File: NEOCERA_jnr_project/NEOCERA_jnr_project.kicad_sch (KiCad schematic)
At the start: 2 parts, among them J4 DB25_Receptacle_MountingHoles, J5 DA15_Receptacle_MountingHoles

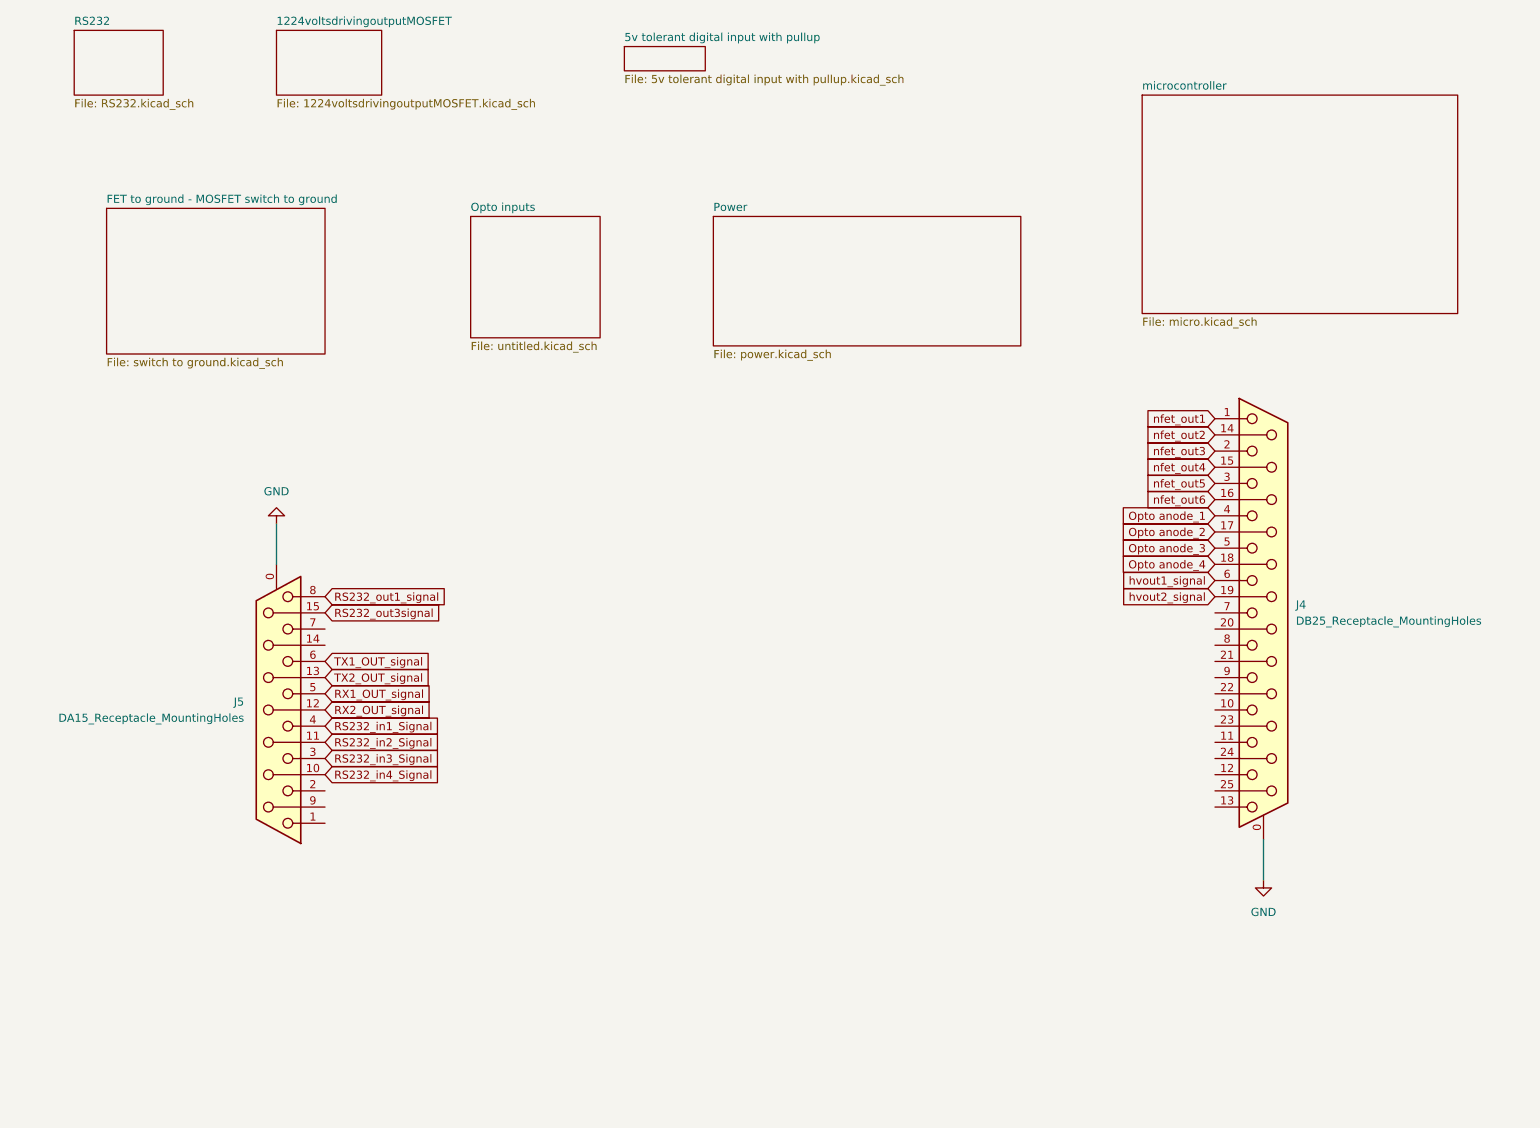
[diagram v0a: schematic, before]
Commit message: bunch of edits
bunch of edits were done including DB37
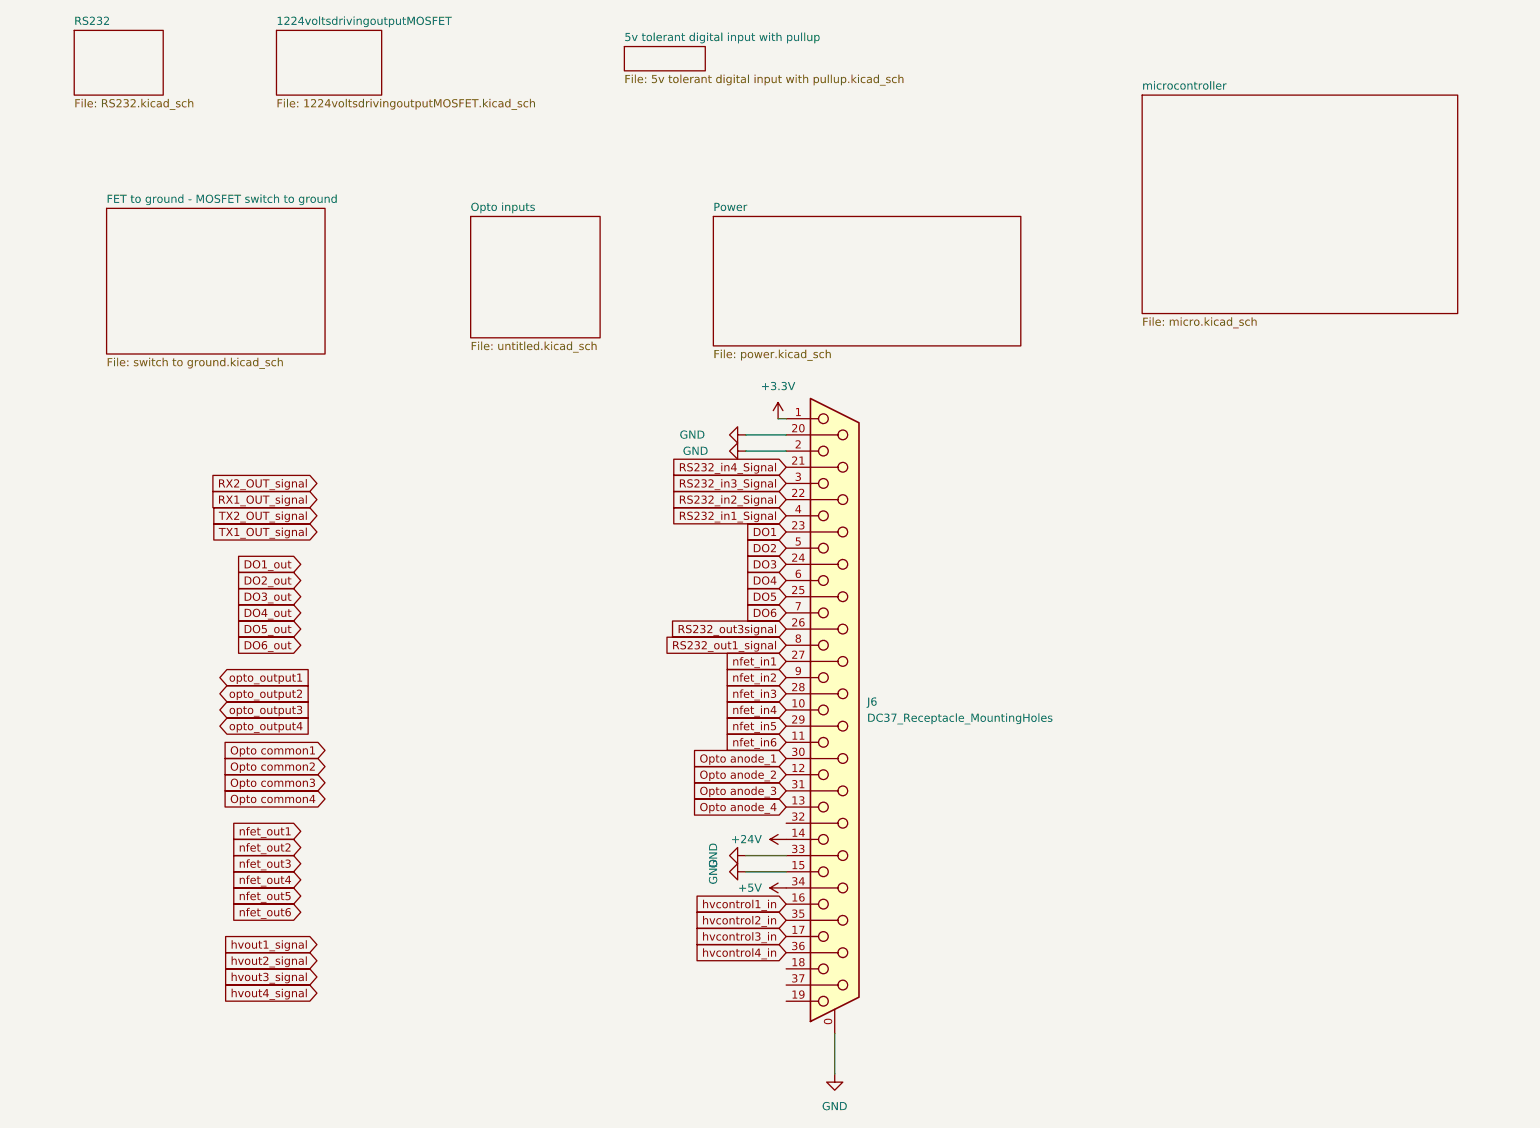
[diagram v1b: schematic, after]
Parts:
- removed J4: DB25_Receptacle_MountingHoles, symbol Connector:DB25_Receptacle_MountingHoles
- removed J5: DA15_Receptacle_MountingHoles, symbol Connector:DA15_Receptacle_MountingHoles
- added J6: DC37_Receptacle_MountingHoles, symbol Connector:DC37_Receptacle_MountingHoles
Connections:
- net GND: now also J6.0 (PAD), J6.15, J6.2, J6.20, J6.33
- net Opto anode_1: now also J6.30
- net Opto anode_2: now also J6.12
- net Opto anode_3: now also J6.31
- net Opto anode_4: now also J6.13
- net RS232_in1_Signal: now also J6.4
- net RS232_in2_Signal: now also J6.22
- net RS232_in3_Signal: now also J6.3
- net RS232_in4_Signal: now also J6.21
- net RS232_out1_signal: now also J6.8
- net RS232_out3signal: now also J6.26
- new net +24V: J6.14
- new net +3.3V: J6.1
- new net +5V: J6.34
- new net DO1: J6.23
- new net DO2: J6.5
- new net DO3: J6.24
- new net DO4: J6.6
- new net DO5: J6.25
- new net DO6: J6.7
- new net hvcontrol1_in: J6.16
- new net hvcontrol2_in: J6.35
- new net hvcontrol3_in: J6.17
- new net hvcontrol4_in: J6.36
- new net nfet_in1: J6.27
- new net nfet_in2: J6.9
- new net nfet_in3: J6.28
- new net nfet_in4: J6.10
- new net nfet_in5: J6.29
- new net nfet_in6: J6.11

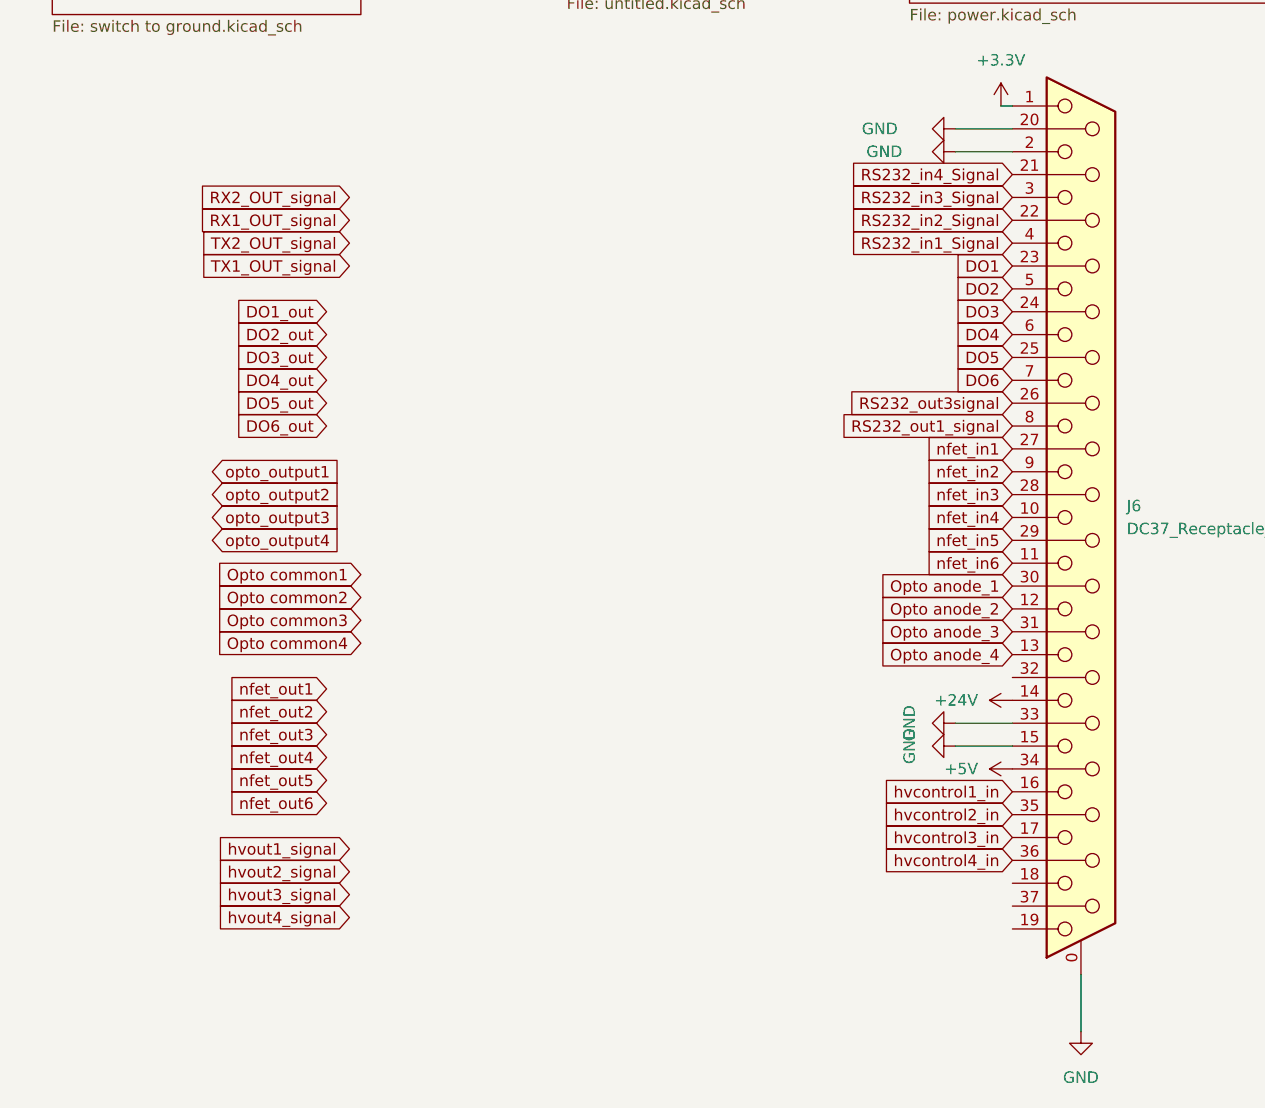
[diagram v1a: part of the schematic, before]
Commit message: bunch
bunch
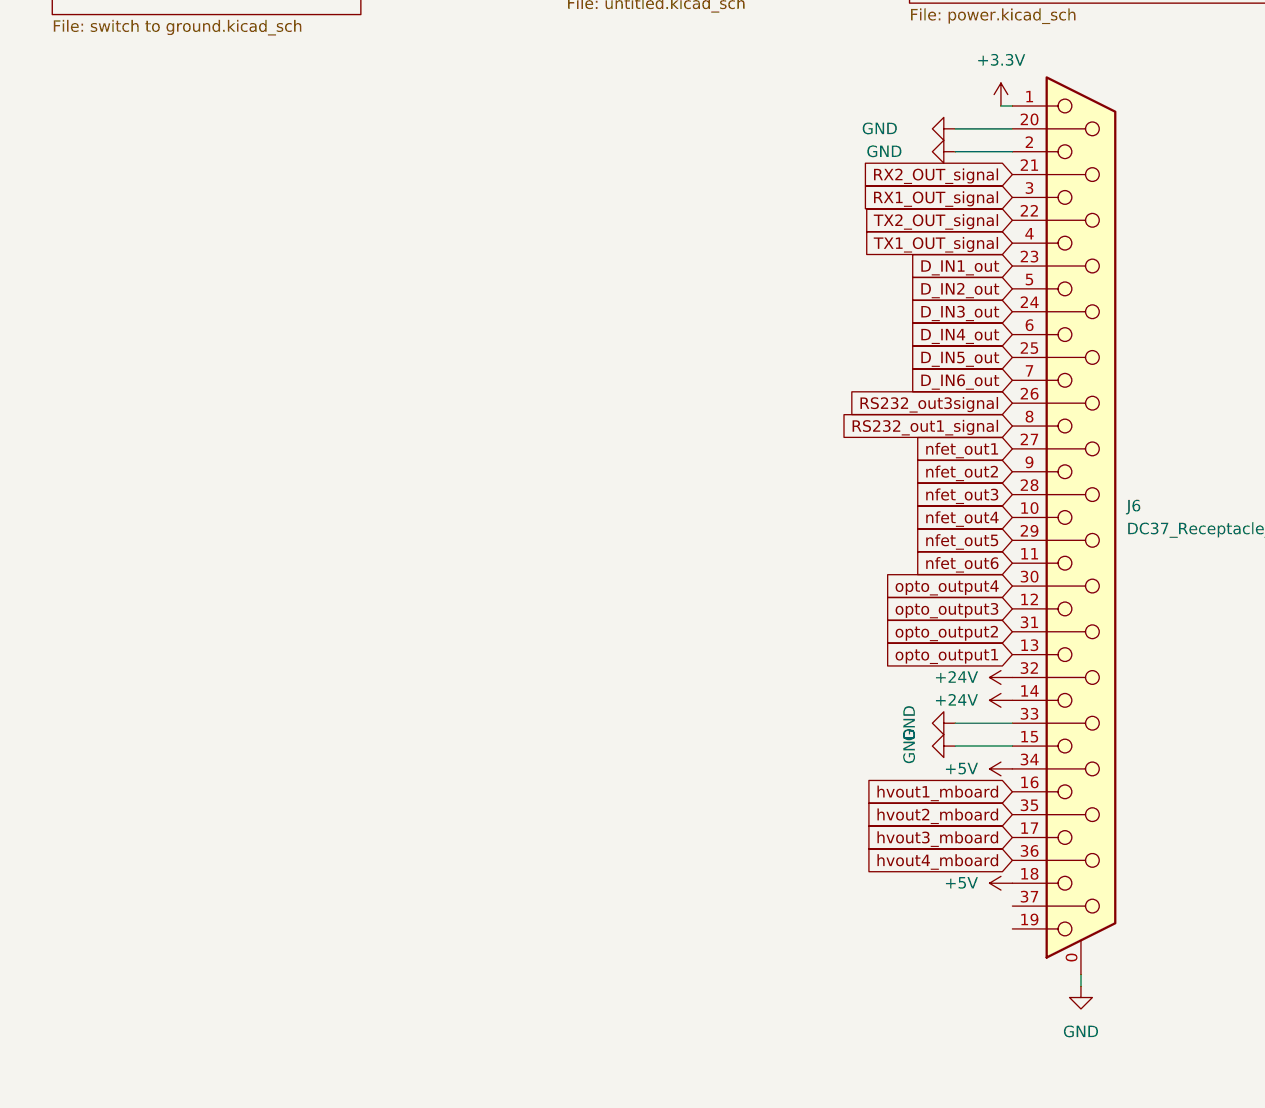
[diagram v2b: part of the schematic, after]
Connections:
- net Opto anode_1 is gone; now on net opto_output4: J6.30
- net Opto anode_2 is gone; now on net opto_output3: J6.12
- net Opto anode_3 is gone; now on net opto_output2: J6.31
- net Opto anode_4 is gone; now on net opto_output1: J6.13
- net RS232_in1_Signal is gone; now on net TX1_OUT_signal: J6.4
- net RS232_in2_Signal is gone; now on net TX2_OUT_signal: J6.22
- net RS232_in3_Signal is gone; now on net RX1_OUT_signal: J6.3
- net RS232_in4_Signal is gone; now on net RX2_OUT_signal: J6.21
- net nfet_in1 is gone; now on net nfet_out1: J6.27
- net nfet_in2 is gone; now on net nfet_out2: J6.9
- net nfet_in3 is gone; now on net nfet_out3: J6.28
- net nfet_in4 is gone; now on net nfet_out4: J6.10
- net nfet_in5 is gone; now on net nfet_out5: J6.29
- net nfet_in6 is gone; now on net nfet_out6: J6.11
- net +24V: now also J6.32
- net +5V: now also J6.18
- net DO1 renamed D_IN1_out
- net DO2 renamed D_IN2_out
- net DO3 renamed D_IN3_out
- net DO4 renamed D_IN4_out
- net DO5 renamed D_IN5_out
- net DO6 renamed D_IN6_out
- net hvcontrol1_in renamed hvout1_mboard
- net hvcontrol2_in renamed hvout2_mboard
- net hvcontrol3_in renamed hvout3_mboard
- net hvcontrol4_in renamed hvout4_mboard
